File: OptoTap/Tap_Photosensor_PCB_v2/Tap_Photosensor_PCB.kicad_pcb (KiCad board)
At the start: 2 copper layers, 28.8 x 14.3 mm, 12 parts, among them J1 Conn_01x03, U1 OPB961N51, U2 AP63205WU

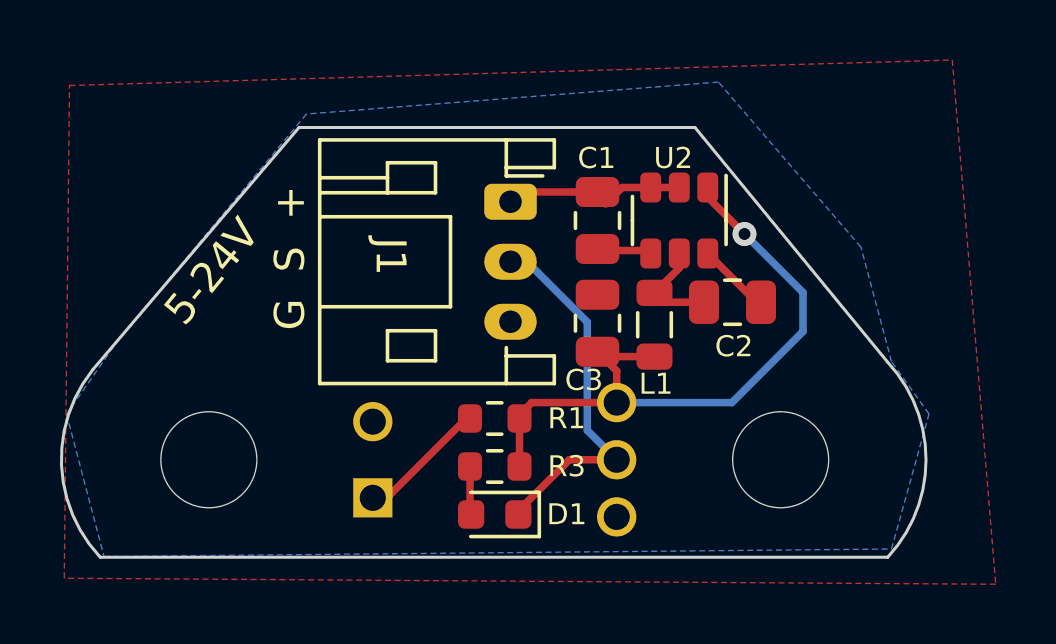
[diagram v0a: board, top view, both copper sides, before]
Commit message: updated OptoTap boards
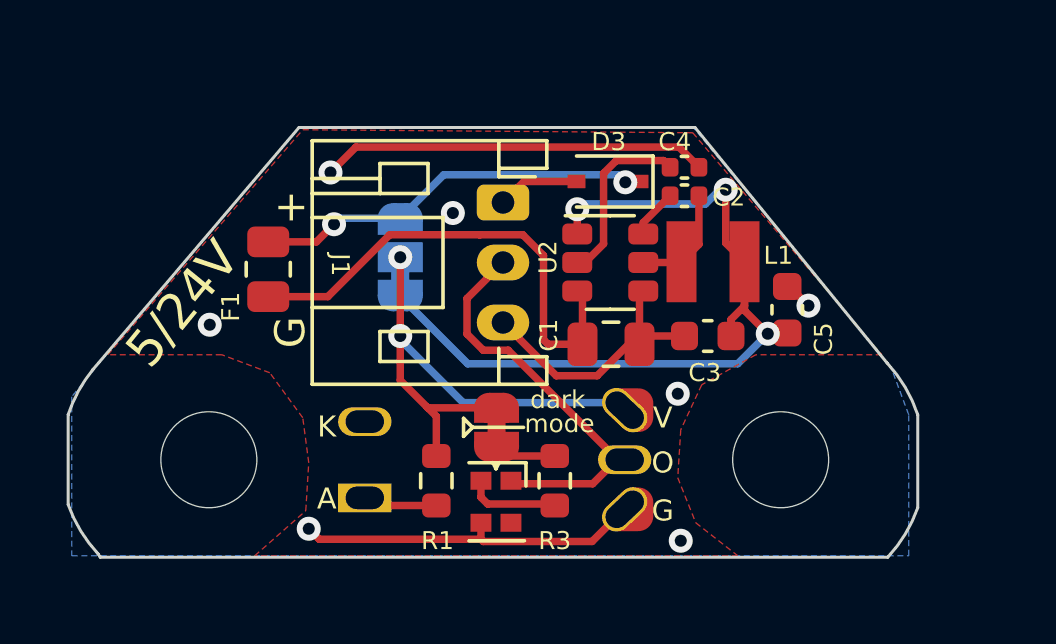
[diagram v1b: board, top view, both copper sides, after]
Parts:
- added C4: 68 nF, Capacitor_SMD:C_0402_1005Metric, F.Cu at (118.7, 55.8)
- added C5: 22 µF, Capacitor_SMD:C_0603_1608Metric, F.Cu at (122.2, 60.5)
- added D3: D_Schottky, Diode_SMD:D_SOD-323, F.Cu at (116.2, 56.2)
- added F1: Polyfuse_Small, Resistor_SMD:R_0805_2012Metric, F.Cu at (104.8, 59.1)
- added JP1: SolderJumper_3_Bridged12, Jumper:SolderJumper-3_P1.3mm_Bridged12_RoundedPad1.0x1.5mm_NumberLabels, B.Cu at (109.2, 58.8)
- added JP2: SolderJumper_2_Bridged, Jumper:SolderJumper-2_DARKMODE, F.Cu at (112.5, 64.4)
- C2: value 220 nF -> 100 nF; footprint Capacitor_SMD:C_0805_2012Metric -> Capacitor_SMD:C_0402_1005Metric
- C3: footprint Capacitor_SMD:C_0805_2012Metric -> Capacitor_SMD:C_0603_1608Metric
- D1: value LED -> XL-1615RGBC; footprint LED_SMD:LED_0603_1608Metric -> LED_SMD:LED_0606_1432
- L1: footprint Inductor_SMD:L_0805_2012Metric -> Inductor_SMD:CKCS3010
- R3: value 640R -> 620R
- U1: footprint footprints:OPTO_OPB961N51 -> footprints:OPTO_EE-SX398_OPB666N
- moved C1 4.15 mm to (116.3, 61.6), turned to 0 degrees
- moved C2 3.89 mm to (118.7, 56.7), turned to 180 degrees
- moved C3 3.70 mm to (119.5, 61.4), turned to 180 degrees
- moved L1 2.87 mm to (119.7, 58.9), turned to 0 degrees
- moved R1 2.85 mm to (110.5, 66.2), turned to -90 degrees
- moved U2 2.69 mm to (116.2, 58.9), turned to 0 degrees
- moved R3 2.06 mm to (114.4, 66.2), turned to -90 degrees
- moved D1 0.43 mm to (112.4, 66.9), turned to -90 degrees
- moved J1 0.25 mm to (112.7, 56.9)
- turned U1 to 180 degrees
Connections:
- net Net-(C2-Pad1) renamed /sw_node
- net Net-(C2-Pad2) renamed /bst
- C1 pad 1: Vin -> /fuse_out
- C3 pad 1: +5V -> /fb
- L1 pad 2: +5V -> /fb
- R3 pad 1: +5V -> Net-(JP2-A)
- U2 pad 1: +5V -> /fb
- U2 pad 2: Vin -> Net-(U2-EN)
- U2 pad 3: Vin -> /fuse_out
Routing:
- net GND: track 1.95 -> 35.8 mm, vias 0 -> 7
- net /fb: track 0.00 -> 27.7 mm, vias 0 -> 3
- net /fuse_out: track 0.00 -> 16.3 mm
- net Vcc: track 0.00 -> 13.4 mm, vias 0 -> 2
- net Net-(U2-EN): track 0.00 -> 5.97 mm
- net +5V: track 22.2 -> 17.6 mm, vias 1 -> 2
- net Vin: track 5.77 -> 2.74 mm
- net Net-(U1-ANODE): track 4.39 -> 2.22 mm
- net Net-(JP2-A): track 0.00 -> 2.07 mm
- net Net-(D1-A): track 1.62 -> 3.12 mm
- net SIG: track 12.4 -> 13.5 mm
- net /bst: track 2.45 -> 1.65 mm
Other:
- board size 28.8 x 14.3 mm -> 28.3 x 14.3 mm
- board text added: "5/24V"
- board text added: "5V 24V"
- board text added: "G +"
- board text added: "OptoTap"
- board text added: "cut trace to change"
- board text added: "rev 2.4.1"
- board text removed: "5-24V"
- board text removed: "5-24V OK"
- board text removed: "G S +"
- board text removed: "OPB666N"
- board text removed: "OptoTap PCB"
- board text removed: "rev 2.1"
